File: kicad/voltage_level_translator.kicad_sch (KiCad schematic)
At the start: 20 parts, among them Q1 2N7002, Q2 2N7002, Q3 2N7002, U3 TMUX1574PW, U4 LSF0108PW, U5 LSF0108PW, U6 LSF0108PW, U7 TMUX1574PW, U8 TXS0108EPW, U9 TXS0108EPW

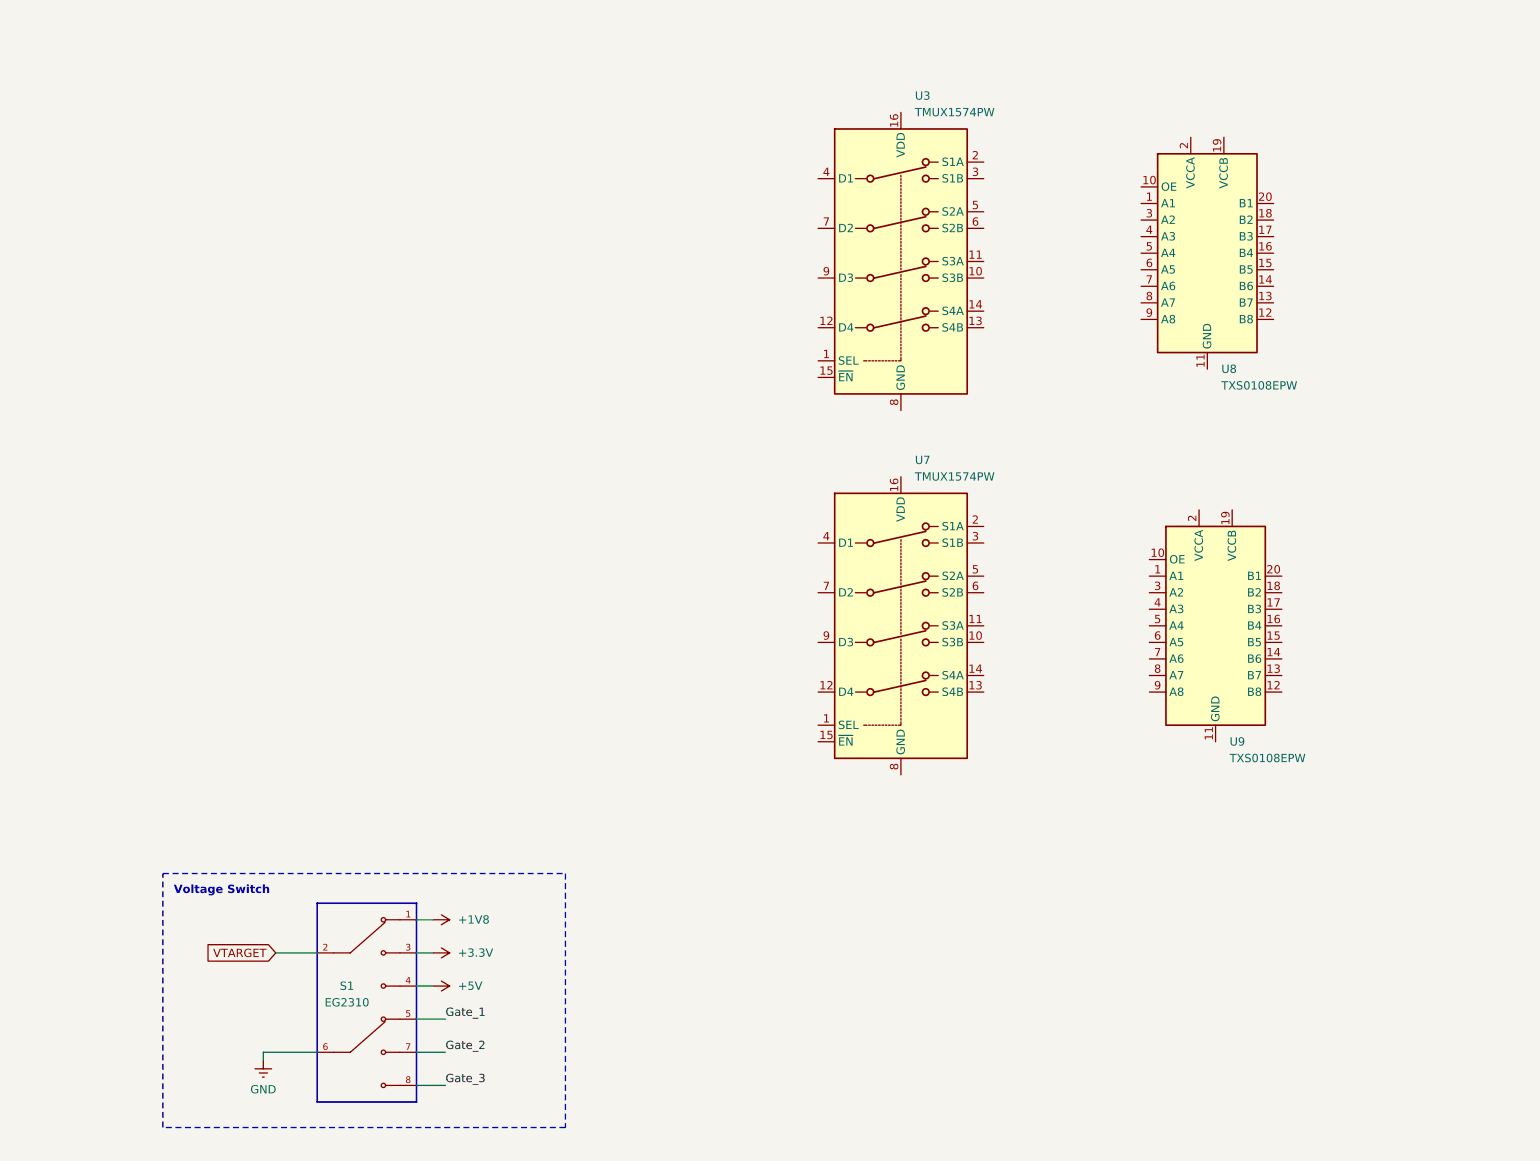
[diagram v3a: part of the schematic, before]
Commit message: Update voltage_level_translator.kicad_sch
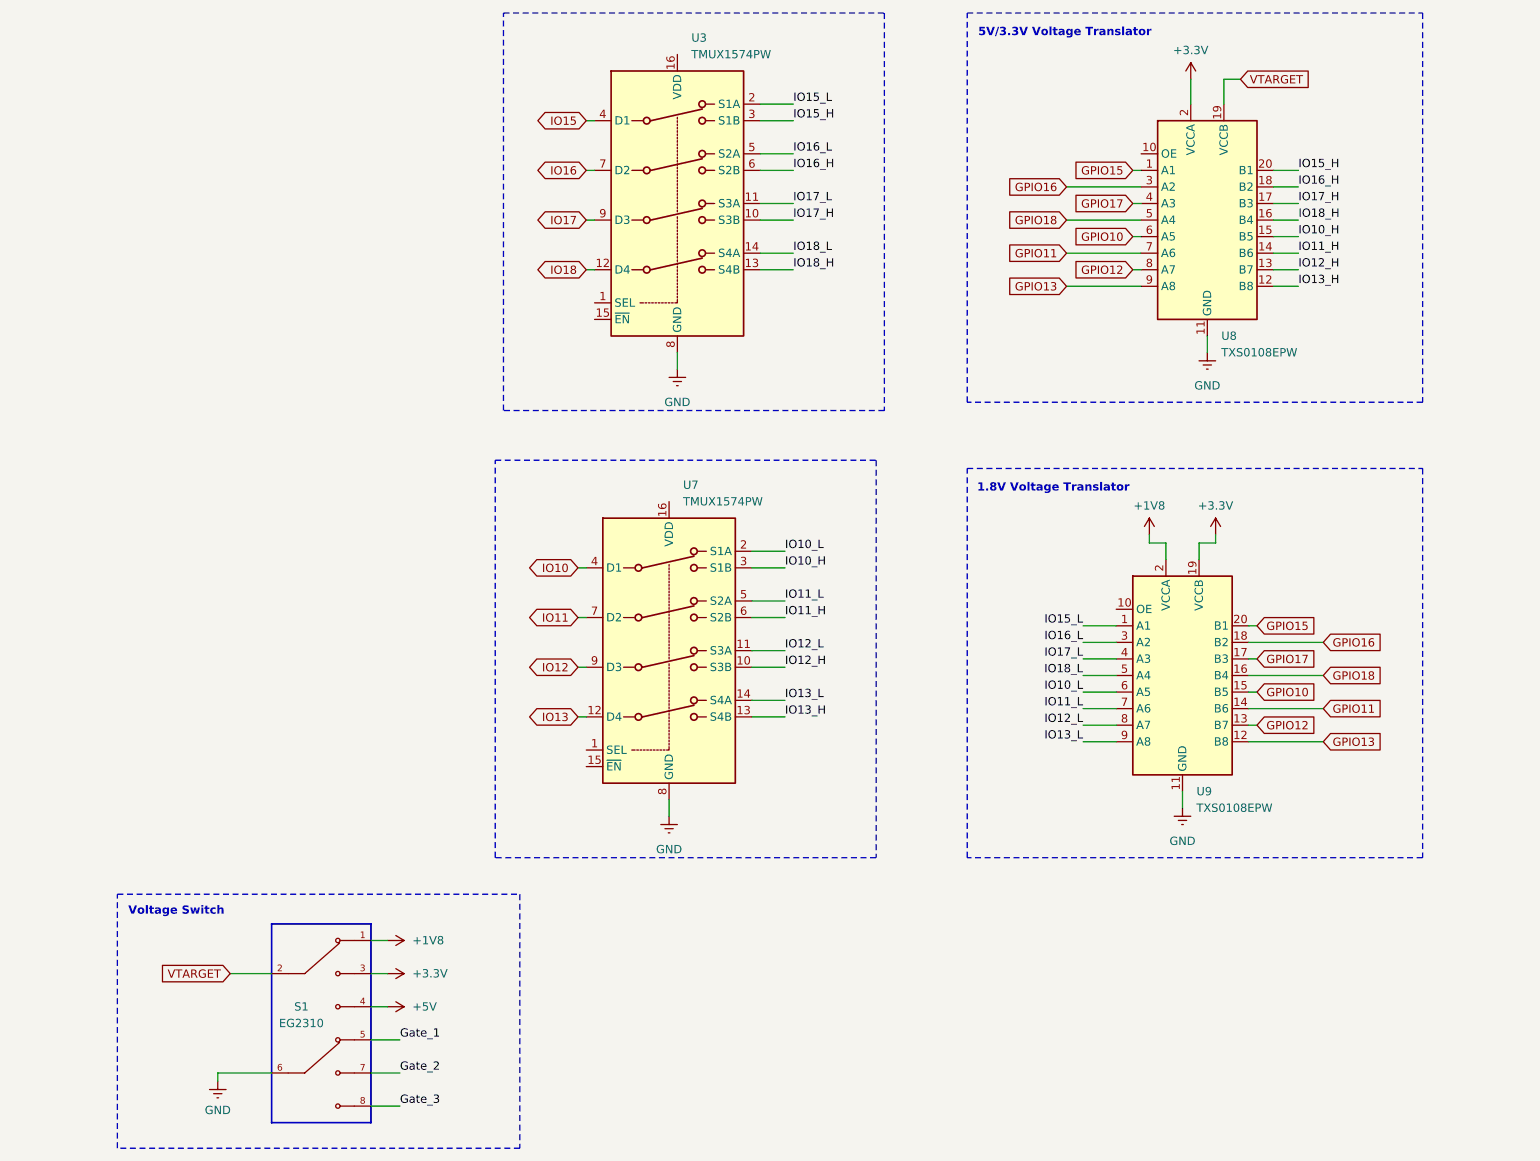
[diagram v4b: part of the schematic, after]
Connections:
- net +1V8: now also U9.2 (VCCA)
- net +3.3V: now also U8.2 (VCCA), U9.19 (VCCB)
- net GND: now also U3.8 (GND), U7.8 (GND), U8.11 (GND), U9.11 (GND)
- net GPIO10: now also U8.6 (A5), U9.15 (B5)
- net GPIO11: now also U8.7 (A6), U9.14 (B6)
- net GPIO12: now also U8.8 (A7), U9.13 (B7)
- net GPIO13: now also U8.9 (A8), U9.12 (B8)
- net GPIO15: now also U8.1 (A1), U9.20 (B1)
- net GPIO16: now also U8.3 (A2), U9.18 (B2)
- net GPIO17: now also U8.4 (A3), U9.17 (B3)
- net GPIO18: now also U8.5 (A4), U9.16 (B4)
- net IO10: now also U7.4 (D1)
- net IO11: now also U7.7 (D2)
- net IO12: now also U7.9 (D3)
- net IO13: now also U7.12 (D4)
- net IO15: now also U3.4 (D1)
- net IO16: now also U3.7 (D2)
- net IO17: now also U3.9 (D3)
- net IO18: now also U3.12 (D4)
- net VTARGET: now also U8.19 (VCCB)
- net IO13_H: now reaches U8.12 (B8)
- net IO13_H: now also U7.13 (S4B)
- net IO12_H: now reaches U8.13 (B7)
- net IO12_H: now also U7.10 (S3B)
- net IO11_H: now reaches U8.14 (B6)
- net IO11_H: now also U7.6 (S2B)
- net IO10_H: now reaches U8.15 (B5)
- net IO10_H: now also U7.3 (S1B)
- net IO17_H: now reaches U8.17 (B3)
- net IO17_H: now also U3.10 (S3B)
- net IO16_H: now reaches U8.18 (B2)
- net IO16_H: now also U3.6 (S2B)
- net IO15_H: now reaches U8.20 (B1)
- net IO15_H: now also U3.3 (S1B)
- net IO15_L: now reaches U9.1 (A1)
- net IO15_L: now also U3.2 (S1A)
- net IO16_L: now reaches U9.3 (A2)
- net IO16_L: now also U3.5 (S2A)
- net IO17_L: now reaches U9.4 (A3)
- net IO17_L: now also U3.11 (S3A)
- net IO10_L: now reaches U9.6 (A5)
- net IO10_L: now also U7.2 (S1A)
- net IO11_L: now reaches U9.7 (A6)
- net IO11_L: now also U7.5 (S2A)
- net IO12_L: now reaches U9.8 (A7)
- net IO12_L: now also U7.11 (S3A)
- net IO13_L: now reaches U9.9 (A8)
- net IO13_L: now also U7.14 (S4A)
- net IO18_H: now reaches U3.13 (S4B)
- net IO18_L: now reaches U3.14 (S4A)
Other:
- note added: "5V/3.3V Voltage Translator"
- moved on the sheet: S1, U3, U7, U8, U9
